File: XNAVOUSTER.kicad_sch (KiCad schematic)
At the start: 17 parts, among them J1 xNAV650_J1, J2 DE9_Pins, U1 LM7805_TO220, U2 LM1117-3.3, U3 74LVC2G34 (dual buffer), U4 MAX3232, U5 Ouster OS1

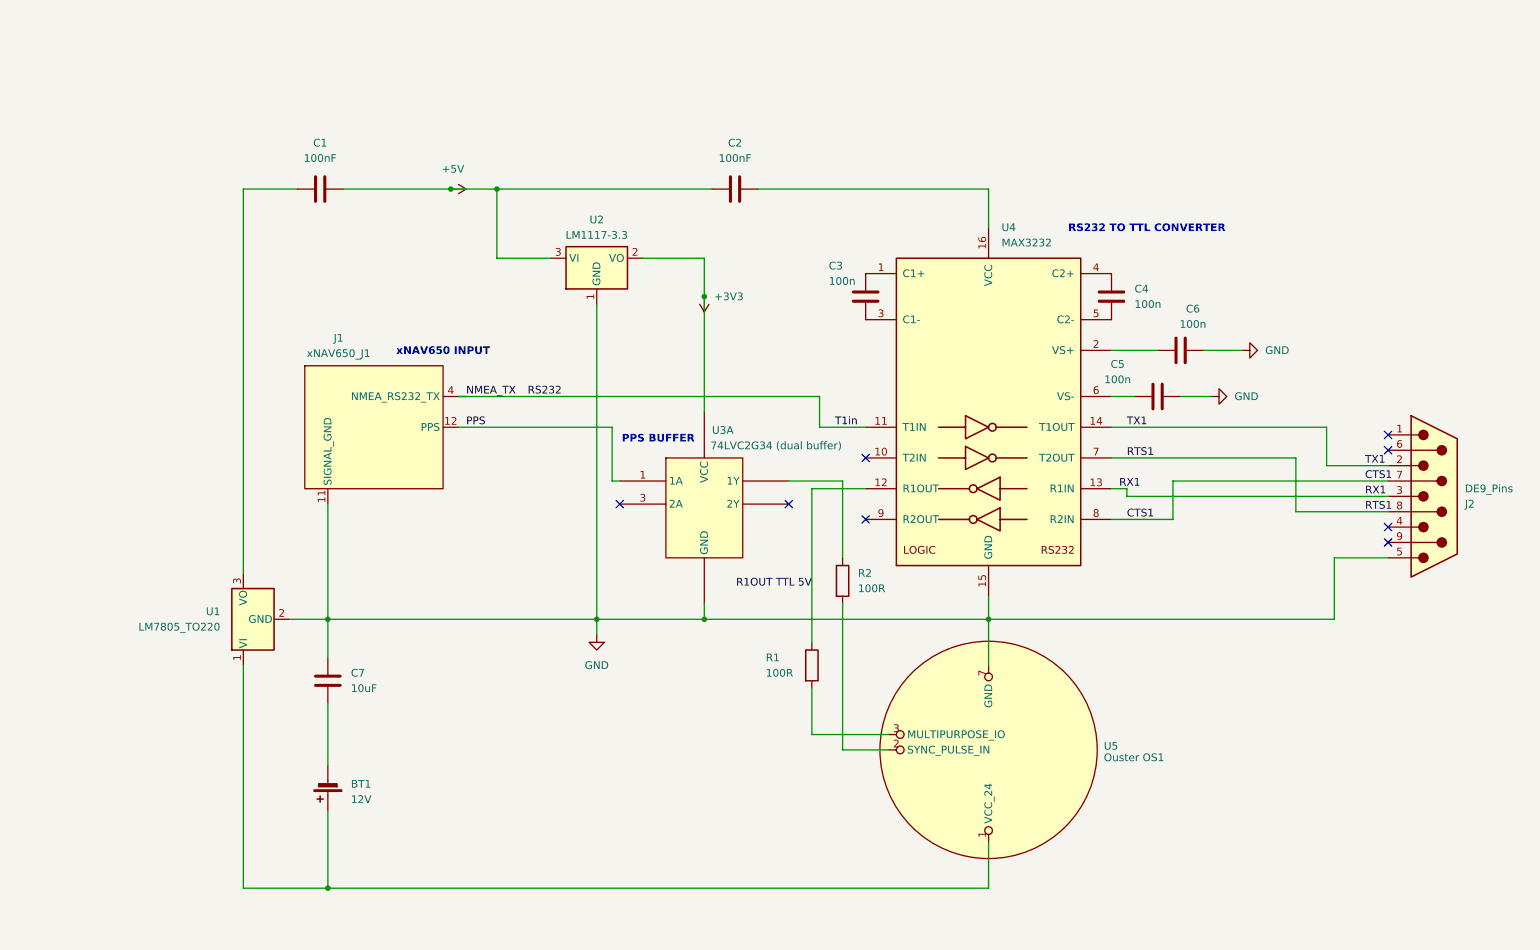
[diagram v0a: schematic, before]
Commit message: commit
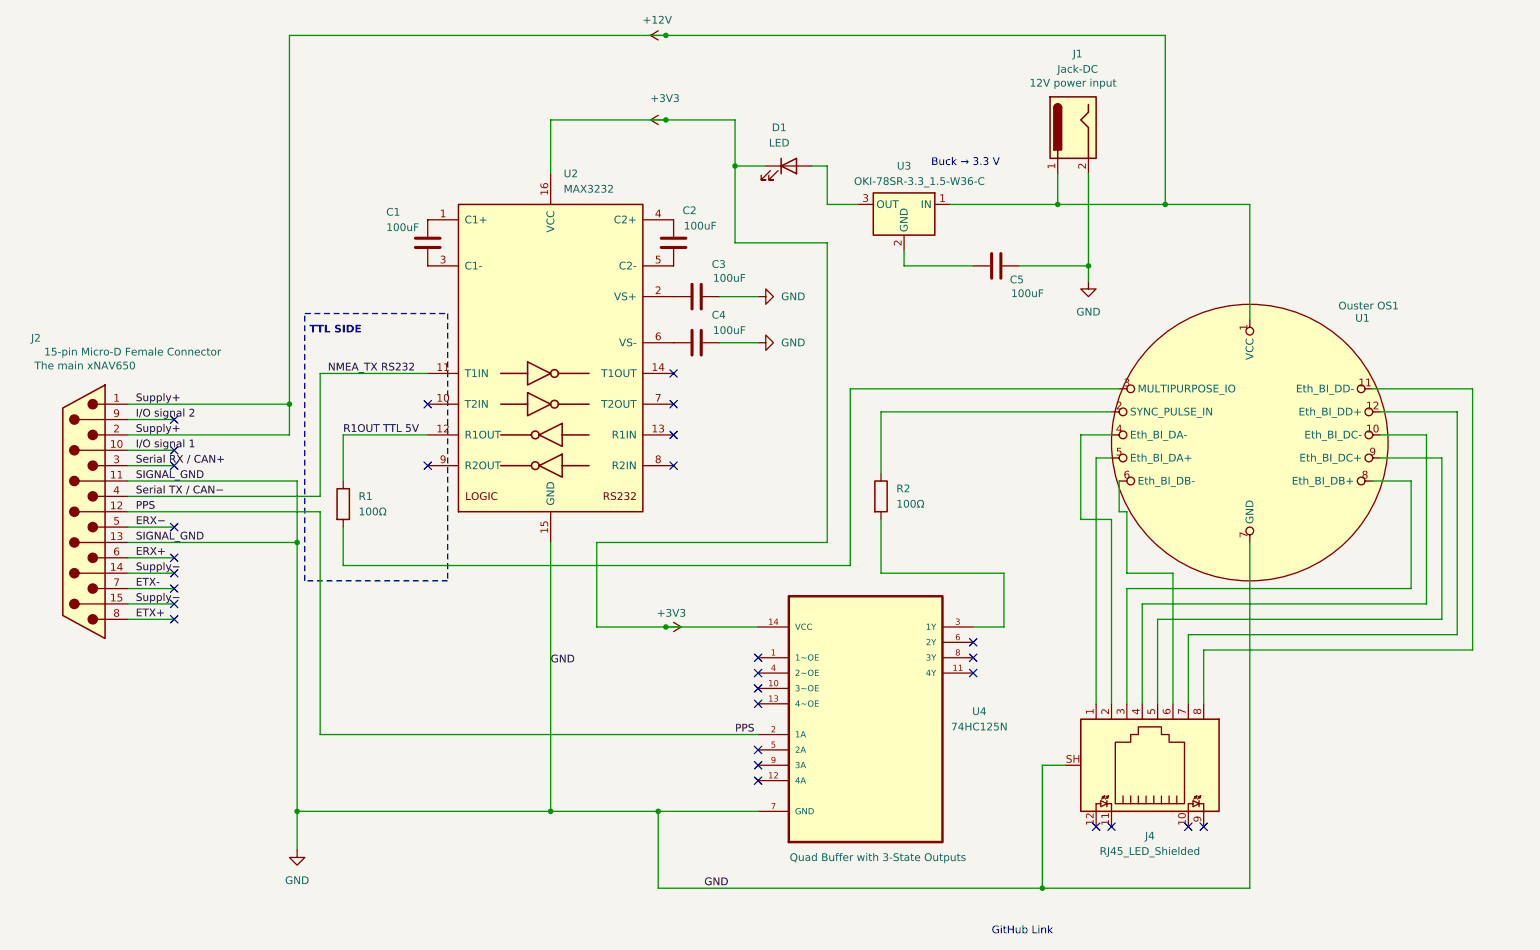
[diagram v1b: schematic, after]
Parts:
- removed BT1: 12V, symbol Device:Battery_Cell
- removed C6: 100n, symbol Device:C
- removed C7: 10uF, symbol Device:C
- removed J1: xNAV650_J1, Connector:Micro-D-15, symbol xNAV650_user_J1_kicad_symbol:xNAV650_user_J1
- removed J2: DE9_Pins, symbol Connector:DE9_Pins
- removed U1: LM7805_TO220, Package_TO_SOT_THT:TO-220-3_Vertical, symbol Regulator_Linear:LM7805_TO220
- removed U2: LM1117-3.3, Package_TO_SOT_SMD:TO-252-3_TabPin2, symbol Regulator_Linear:LM1117DT-3.3
- removed U3: 74LVC2G34 (dual buffer), symbol 74xGxx:74LVC2G34
- removed U4: MAX3232, symbol Interface_UART:MAX3232
- removed U5: Ouster OS1, symbol xNAV650_user_J1_kicad_symbol:OS1
- added D1: LED, LED_THT:LED_D5.0mm, symbol Device:LED
- added J1: Jack-DC, Connector_BarrelJack:BarrelJack_Horizontal, symbol Connector:Jack-DC
- added J2: 15-pin Micro-D Female Connector, Connector_Dsub:DSUB-15_Pins_Horizontal_P2.77x2.84mm_EdgePinOffset7.70mm_Housed_MountingHolesOffset9.12mm, symbol Connector:DA15_Pins
- added J4: RJ45_LED_Shielded, RJ45_Amphenol_54602-x08_Horizontal, symbol Connector:RJ45_LED_Shielded
- added U1: Ouster OS1, symbol xNAV650_user_J1_kicad_symbol:OS1
- added U2: MAX3232, Package_DIP:DIP-16_W7.62mm, symbol Interface_UART:MAX3232
- added U3: OKI-78SR-3.3_1.5-W36-C, Converter_DCDC:Converter_DCDC_Murata_OKI-78SR_Vertical, symbol Converter_DCDC:OKI-78SR-3.3_1.5-W36-C
- added U4: 74HC125N, 74HC125N:DIP254P762X420-14, symbol 74HC125N:74HC125N
- C1, C2: value 100nF -> 100uF; footprint (none) -> Capacitor_THT:CP_Radial_D6.3mm_P2.50mm
- C3, C4, C5: value 100n -> 100uF; footprint (none) -> Capacitor_THT:CP_Radial_D6.3mm_P2.50mm
- R1, R2: value 100R -> 100Ω; footprint (none) -> Resistor_THT:R_Axial_DIN0207_L6.3mm_D2.5mm_P10.16mm_Horizontal
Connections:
- net +3V3: now also D1.1 (K), U2.16 (VCC), U4.14 (VCC)
- net GND: now also C3.2, C4.2, J1.2, J2.11 (P111), J2.13 (P13), J4.SH, U1.7 (GND), U2.15 (GND), U4.7 (GND)
- net PPS: now also J2.12 (P12), U4.2 (1A)
- net R1OUT TTL 5V: now also U2.12 (R1OUT)
- net at R2.2: now also U4.3 (1Y)
- net at R1.2: now also U1.3 (MULTIPURPOSE_IO)
- net at C4.1: now also U2.6 (VS-)
- net at C3.1: now also U2.2 (VS+)
- net at R2.1: now also U1.2 (SYNC_PULSE_IN)
- net at C2.2: now also U2.5 (C2-)
- net at C5.1: now also U3.2 (GND)
- net at C1.1: now also U2.1 (C1+)
- net +5V: no longer names the net of C1.2
- net +5V: now also U2.3 (C1-); no longer C2.1
- new net: J4.1, U1.5 (Eth_BI_DA+)
- new net: J4.2, U1.4 (Eth_BI_DA-)
- new net: J4.3, U1.8 (Eth_BI_DB+)
- new net: J4.4, U1.10 (Eth_BI_DC-)
- new net: J4.5, U1.9 (Eth_BI_DC+)
- new net: J4.6, U1.6 (Eth_BI_DB-)
- new net: J4.7, U1.12 (Eth_BI_DD+)
- new net: J4.8, U1.11 (Eth_BI_DD-)
- new net: C2.1, U2.4 (C2+)
- new net: D1.2 (A), U3.3 (OUT)
- new net +12V: J1.1, J2.1, J2.2, U1.1 (VCC), U3.1 (IN)
- new net ERX+: J2.6
- new net ERX−: J2.5
- new net ETX+: J2.8
- new net ETX-: J2.7
- new net I/O signal 1: J2.10 (P10)
- new net I/O signal 2: J2.9 (P9)
- new net NMEA_TX RS232: J2.4, U2.11 (T1IN)
- new net Serial RX / CAN+: J2.3
- new net Supply−: J2.14 (P14), J2.15 (P15)
- no-connect marks 8 -> 29
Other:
- note added: "Buck → 3.3 V"
- note added: "GitHub Link"
- note added: "TTL SIDE"
- note removed: "PPS BUFFER"
- note removed: "RS232 TO TTL CONVERTER"
- note removed: "xNAV650 INPUT"
- title: xNAV650-OS1-128 -> xNAV650 to Ouster OS1 Adapter
